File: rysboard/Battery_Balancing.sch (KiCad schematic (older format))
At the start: 34 parts, among them J20 Power_SW, J4 Cell3, J5 Cell2, J6 Cell1, Q13 SI7997DP-T1-GE3, Q14 DMP2075UFDB-7-alt, Q9 Si7938DP-T1-GE3, U7 LM74700, U9 INA181

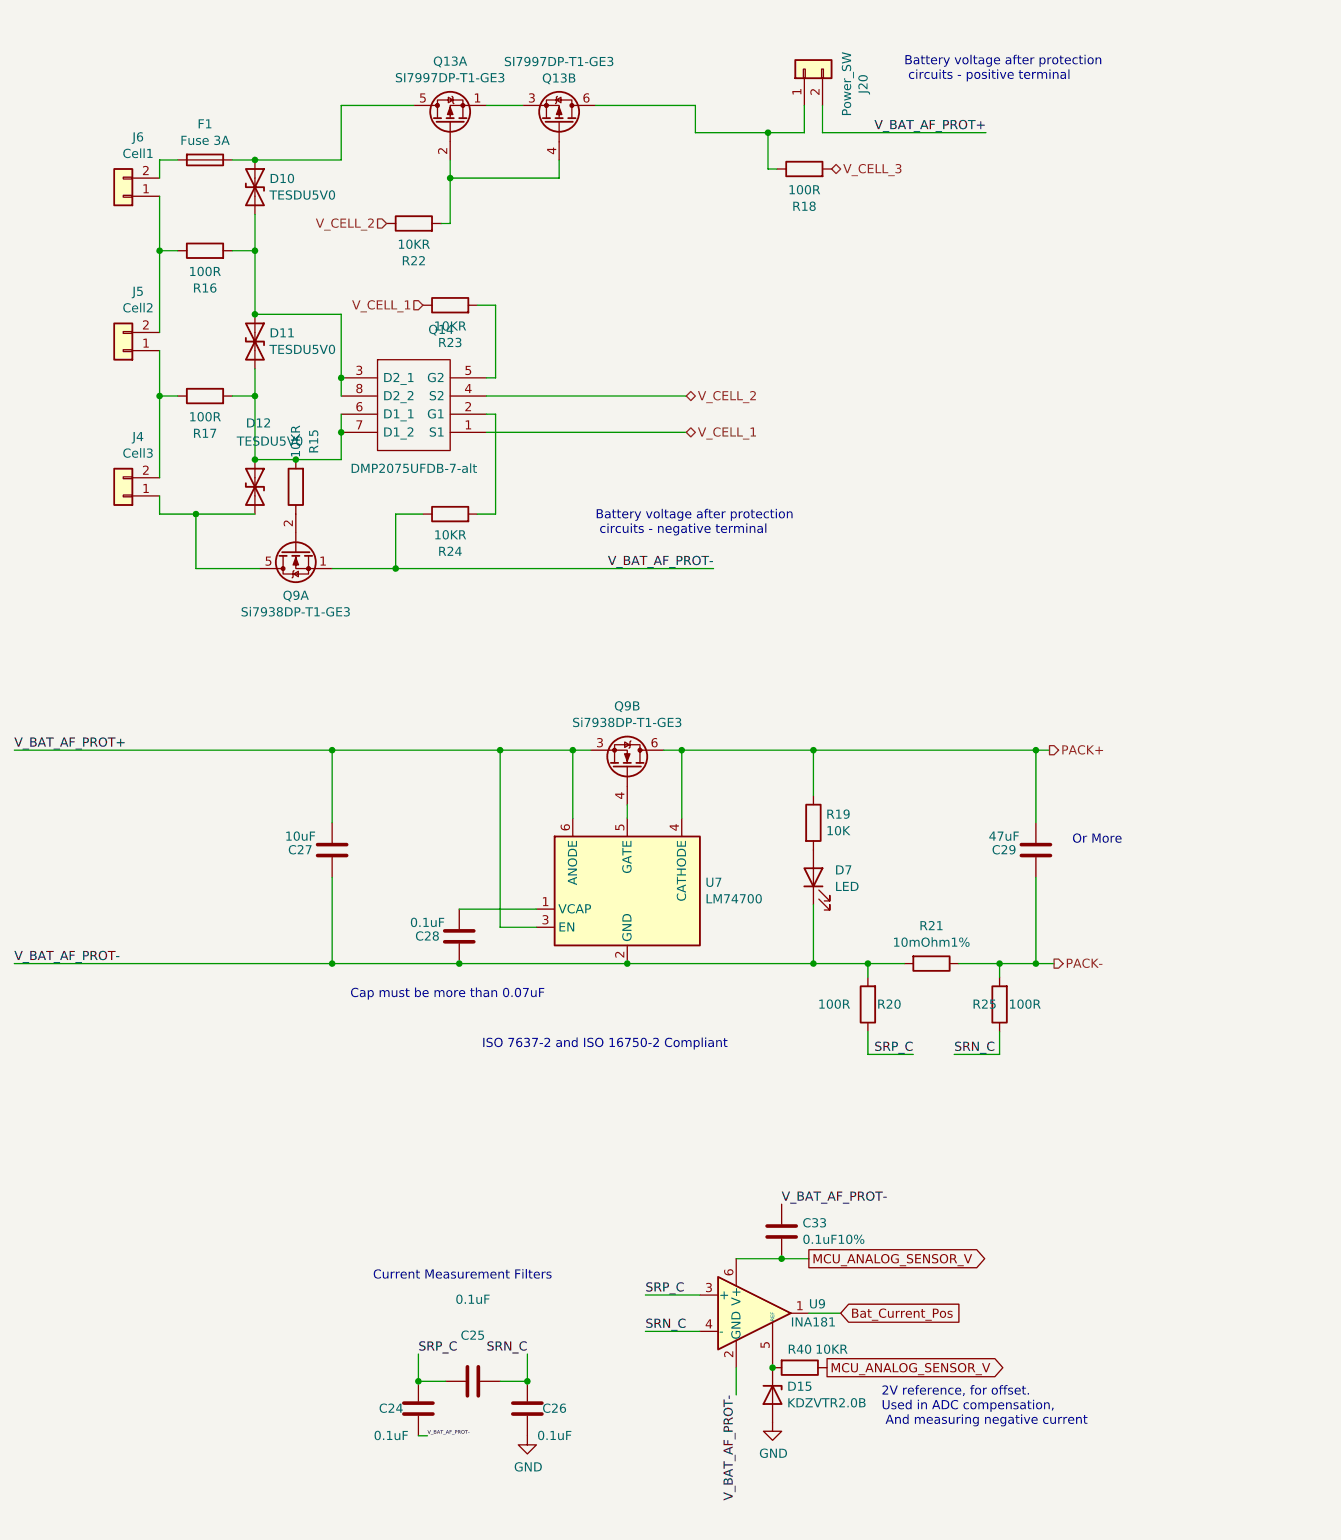
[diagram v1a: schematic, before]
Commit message: Bom finished pcb cleanup started
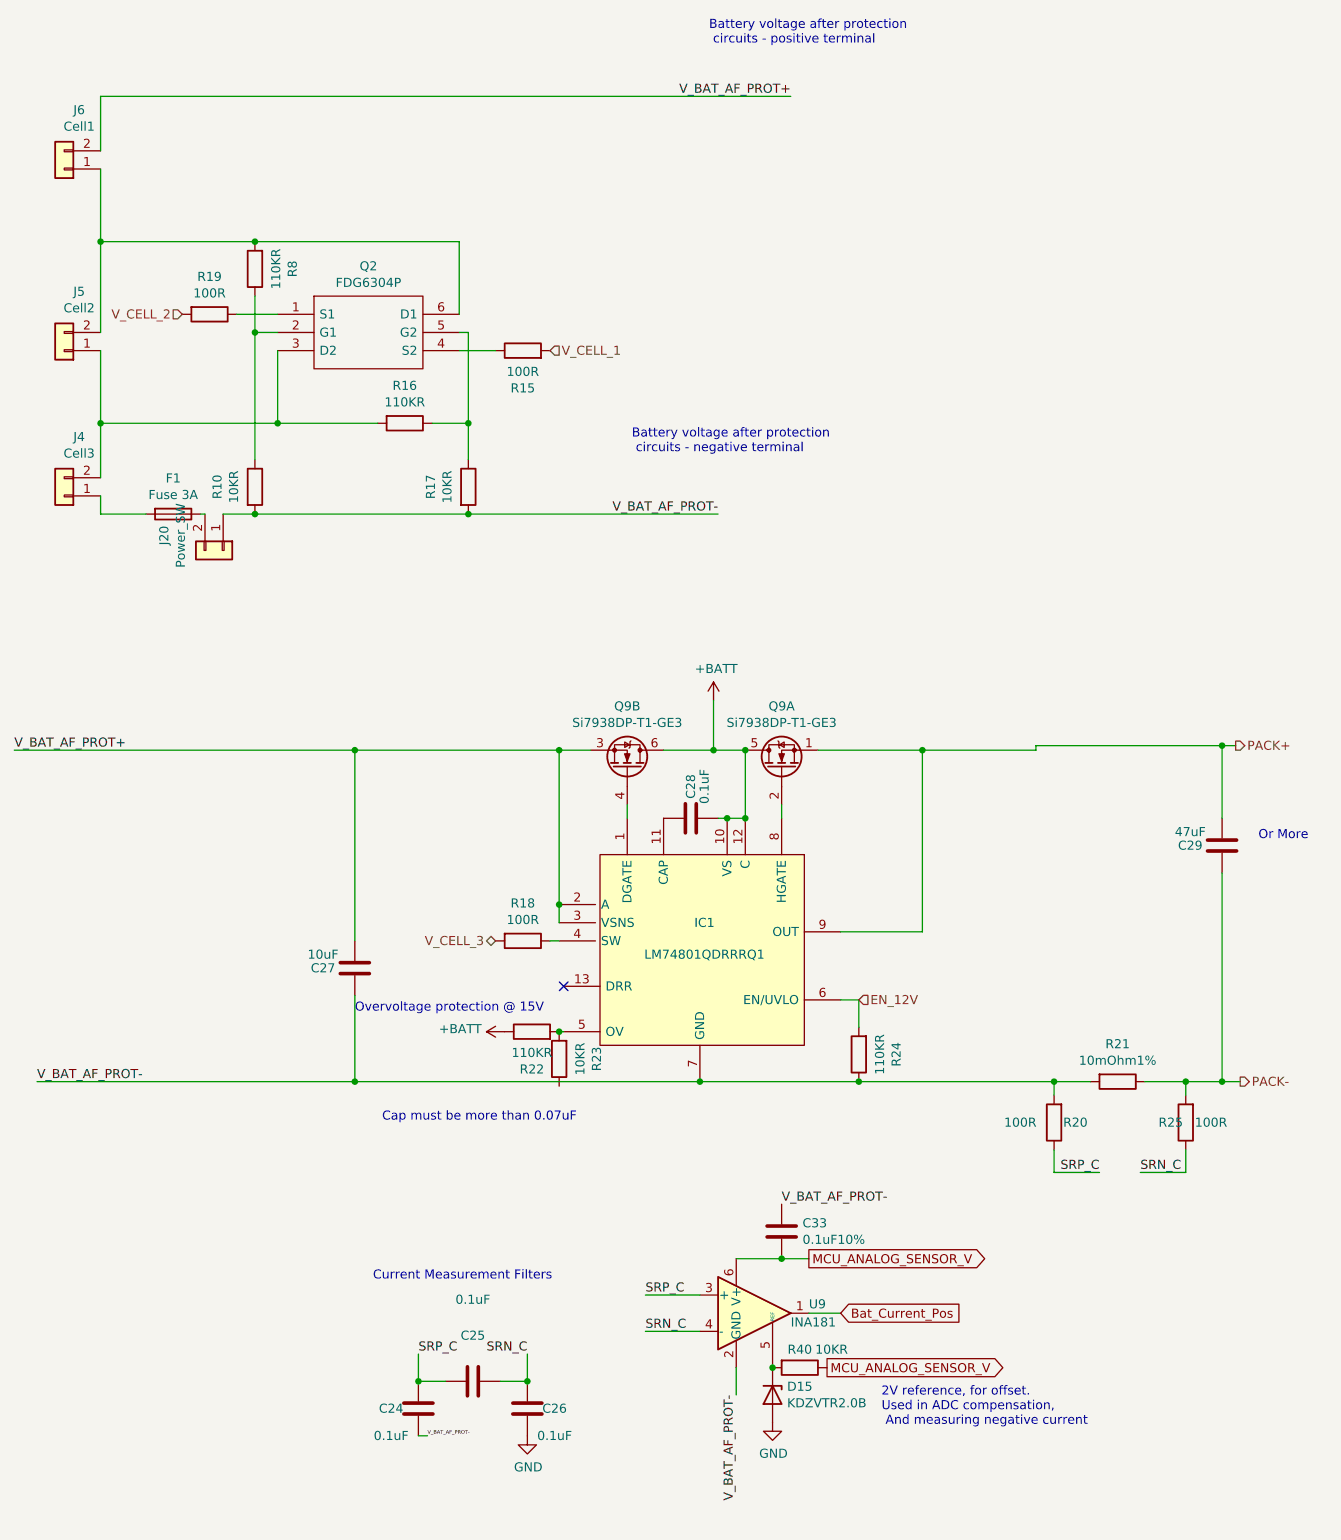
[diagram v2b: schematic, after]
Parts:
- removed D10, D11, D12: TESDU5V0, Diode_SMD:D_0603_1608Metric_Pad1.05x0.95mm_HandSolder, symbol Device:D_TVS
- removed D7: LED, LED_SMD:LED_0805_2012Metric, symbol Device:LED
- removed Q13: SI7997DP-T1-GE3, Package_SO:PowerPAK_SO-8_Dual, symbol rysboard:SI7997DP-T1-GE3
- removed Q14: DMP2075UFDB-7-alt, SamacSys_Parts:DMP2075UFDB7, symbol SamacSys_Parts:DMP2075UFDB-7-alt
- removed U7: LM74700, Package_TO_SOT_SMD:SOT-23-6, symbol Power_Management:LM74700
- added IC1: LM74801QDRRRQ1, LM74801QDRRRQ1, symbol SamacSys_Parts:LM74801QDRRRQ1
- added Q2: FDG6304P, SOT65P210X110-6N, symbol SamacSys_Parts:FDG6304P
- added R10: 10KR, Resistor_SMD:R_0603_1608Metric, symbol Device:R
- added R8: 110KR, Resistor_SMD:R_0603_1608Metric, symbol Device:R
- R15: value 10KR -> 100R
- R16: value 100R -> 110KR
- R17: value 100R -> 10KR
- R19: value 10K -> 100R
- R22, R24: value 10KR -> 110KR
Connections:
- net PACK+: now also Q9.1 (S1), IC1.9 (OUT); no longer Q9.6 (D1), R19.1
- net V_BAT_AF_PROT+: now also J6.2 (Pin_2), IC1.2 (A), IC1.3 (VSNS); no longer J20.2 (Pin_2)
- net V_BAT_AF_PROT-: now also J20.1 (Pin_1), R17.2, IC1.7 (GND), R10.2; no longer C28.1, Q9.1 (S1)
- net V_CELL_1: now also R15.2; no longer R23.1
- net V_CELL_2: now also R19.2; no longer R22.1
- net at J4.1 (Pin_1): now also F1.2; no longer Q9.5 (D1)
- net at J4.2 (Pin_2), J5.1 (Pin_1): now also R16.2, Q2.3 (D2); no longer R17.1
- net at J5.2 (Pin_2), J6.1 (Pin_1): now also Q2.6 (D1), R8.2; no longer R16.1
- net at R18.1: now also IC1.4 (SW); no longer J20.1 (Pin_1)
- net at R15.1: now also Q2.4 (S2); no longer Q9.2 (G1)
- net at F1.1: now also J20.2 (Pin_2)
- net EN_12V: now reaches R24.2
- net EN_12V: now also IC1.6 (EN/UVLO)
- net at R23.2: now also R22.2, IC1.5 (OV)
- net +BATT: now reaches C28.2
- net +BATT: now also Q9.5 (D1), Q9.6 (D1), R22.1, IC1.10 (VS), IC1.12 (C)
- net at Q9.4 (G2): now also IC1.1 (DGATE)
- new net: C28.1, IC1.11 (CAP)
- new net: Q2.1 (S1), R19.1
- new net: IC1.8 (HGATE), Q9.2 (G1)
- new net: Q2.2 (G1), R10.1, R8.1
- new net: Q2.5 (G2), R16.1, R17.1
- no-connect marks 0 -> 1
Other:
- note added: "Overvoltage protection @ 15V"
- note removed: "ISO 7637-2 and ISO 16750-2 Compliant\n"
- moved on the sheet: C27, C28, C29, F1, J20, J4, J5, J6, R18, R20, R21, R25
